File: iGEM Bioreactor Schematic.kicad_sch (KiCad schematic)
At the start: 13 parts, among them M1 Motor_DC, M2 Motor_Servo, Q1 Q_Photo_NPN, U1 L298N, U2 OLED_Display, U3 Pico, U4 DS18B20

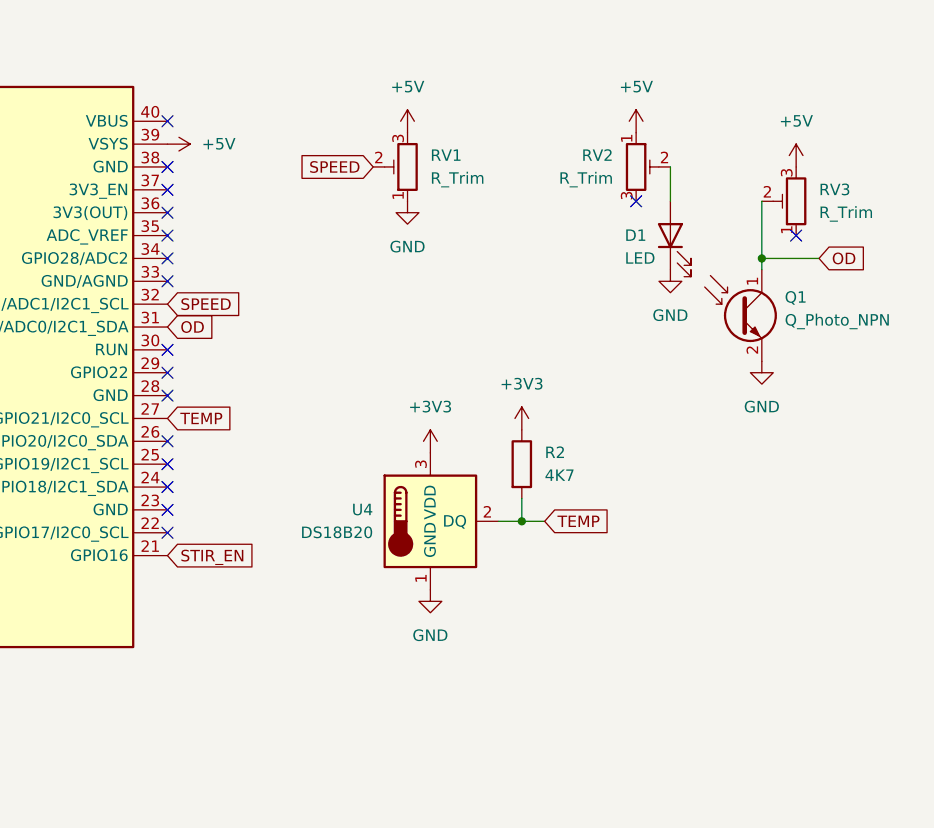
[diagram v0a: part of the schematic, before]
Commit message: Final grow experiments!
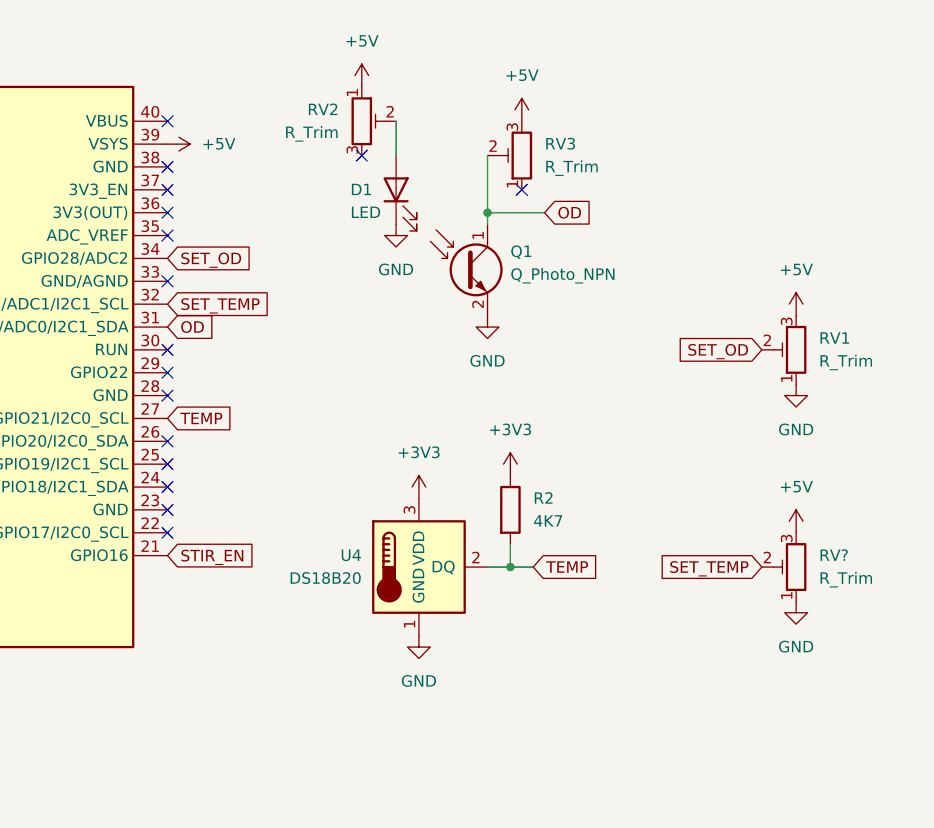
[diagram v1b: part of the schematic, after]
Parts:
- added RV?: R_Trim, symbol Device:R_Potentiometer_Trim
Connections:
- net +5V: now also RV?.3
- net GND: now also RV?.1
- net SET_OD: now reaches U3.34 (GPIO28/ADC2)
- net SET_OD: now also RV1.2
- net SPEED renamed SET_TEMP
- net SET_TEMP: now also RV?.2; no longer RV1.2
- no-connect marks 32 -> 31
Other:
- moved on the sheet: D1, Q1, R2, RV1, RV2, RV3, U4
